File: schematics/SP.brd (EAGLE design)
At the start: 45.6 x 46 mm, 24 parts

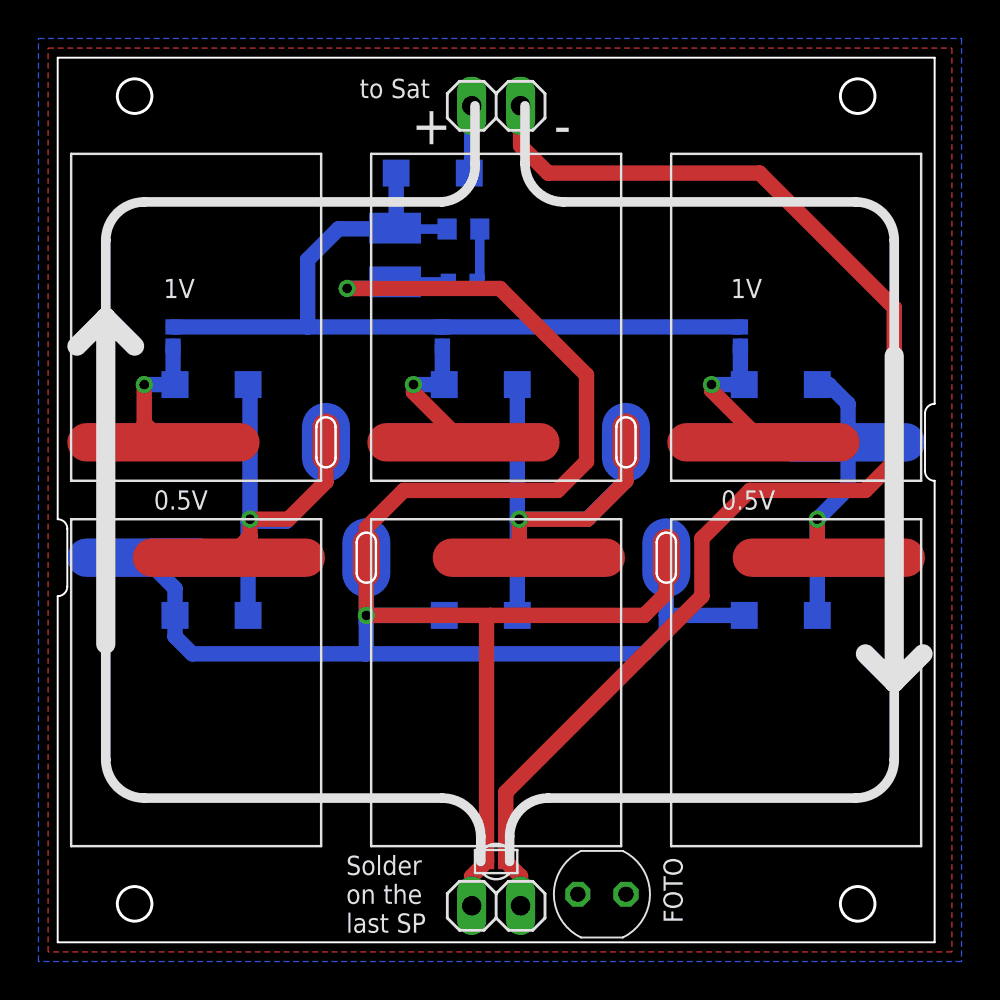
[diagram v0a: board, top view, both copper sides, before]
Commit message: проверка плат
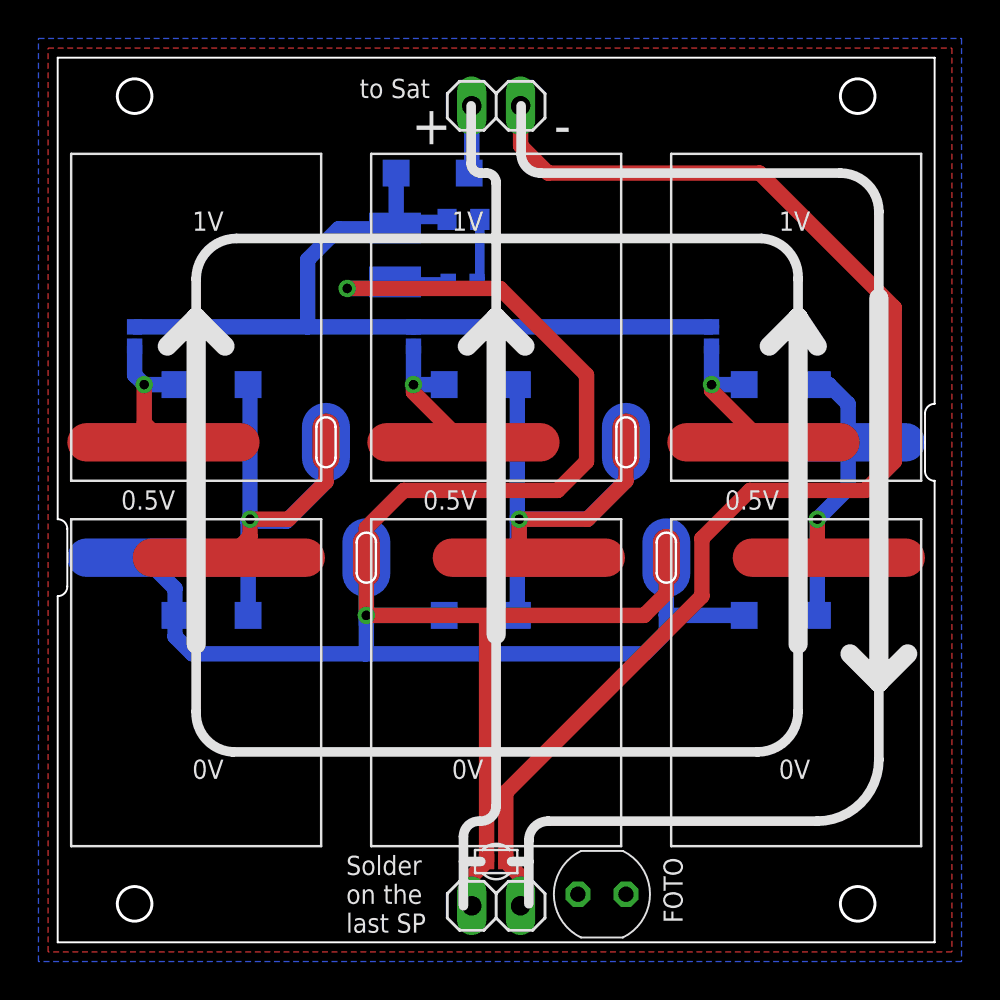
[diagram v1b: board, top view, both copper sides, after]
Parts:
- moved U$5 12.1 mm to (18.5, 4.50)
- moved U$9 2.00 mm to (4.00, 31.5)
- moved U$10 1.50 mm to (18.5, 31.5)
- moved U$11 1.50 mm to (34.0, 31.5)
- moved R1 0.50 mm to (21.1, 37.6)
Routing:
- net SP+: track 43.9 -> 44.6 mm
- net N$4: track 2.78 -> 3.28 mm
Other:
- board text added: "0V"
